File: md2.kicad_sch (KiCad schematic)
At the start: 39 parts, among them IC1 TC74HC4066AP_F_, IC2 TC74HC4066AP_F_, IC3 TC74HC04AP, IC4 TB6643KQ, IC5 TB6643KQ, IC6 TB6643KQ, IC7 TB6643KQ, J1 Conn_01x03_Pin, J10 Conn_01x02_Pin, J11 Conn_01x01_Pin, J2 Conn_01x03_Pin, J3 Conn_01x03_Pin, J4 Conn_01x03_Pin, J5 XT30PW-M, J6 XT30PW-M, J7 XT30PW-M, J8 XT30PW-M, J9 Conn_01x02_Pin, SW1 SW_Push, SW2 SW_Push, SW3 SW_Push, SW4 SW_Push, SW5 SW_Push, SW6 SW_Push, SW7 SW_Push, SW8 SW_Push, SW9 SW_Push, U1 NJM7805FA

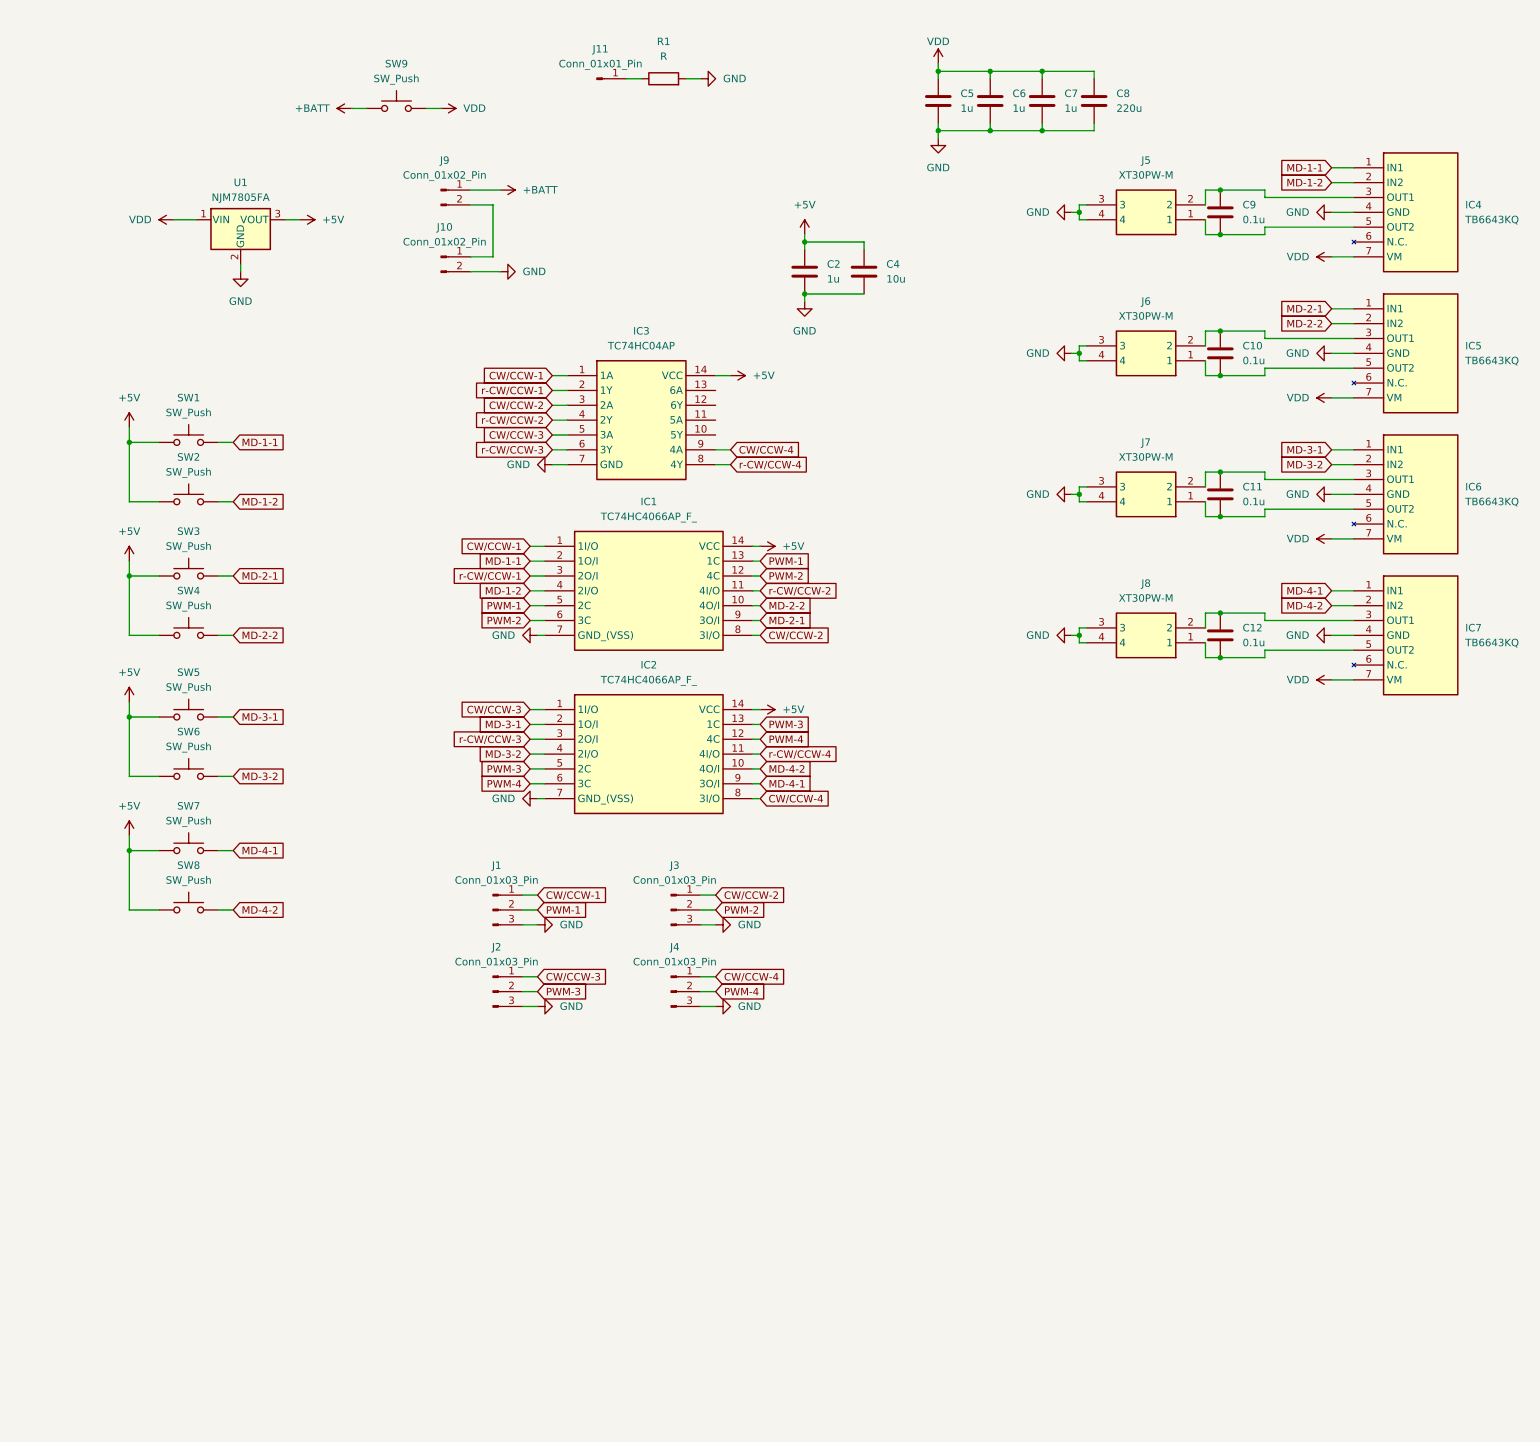
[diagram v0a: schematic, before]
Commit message: Update
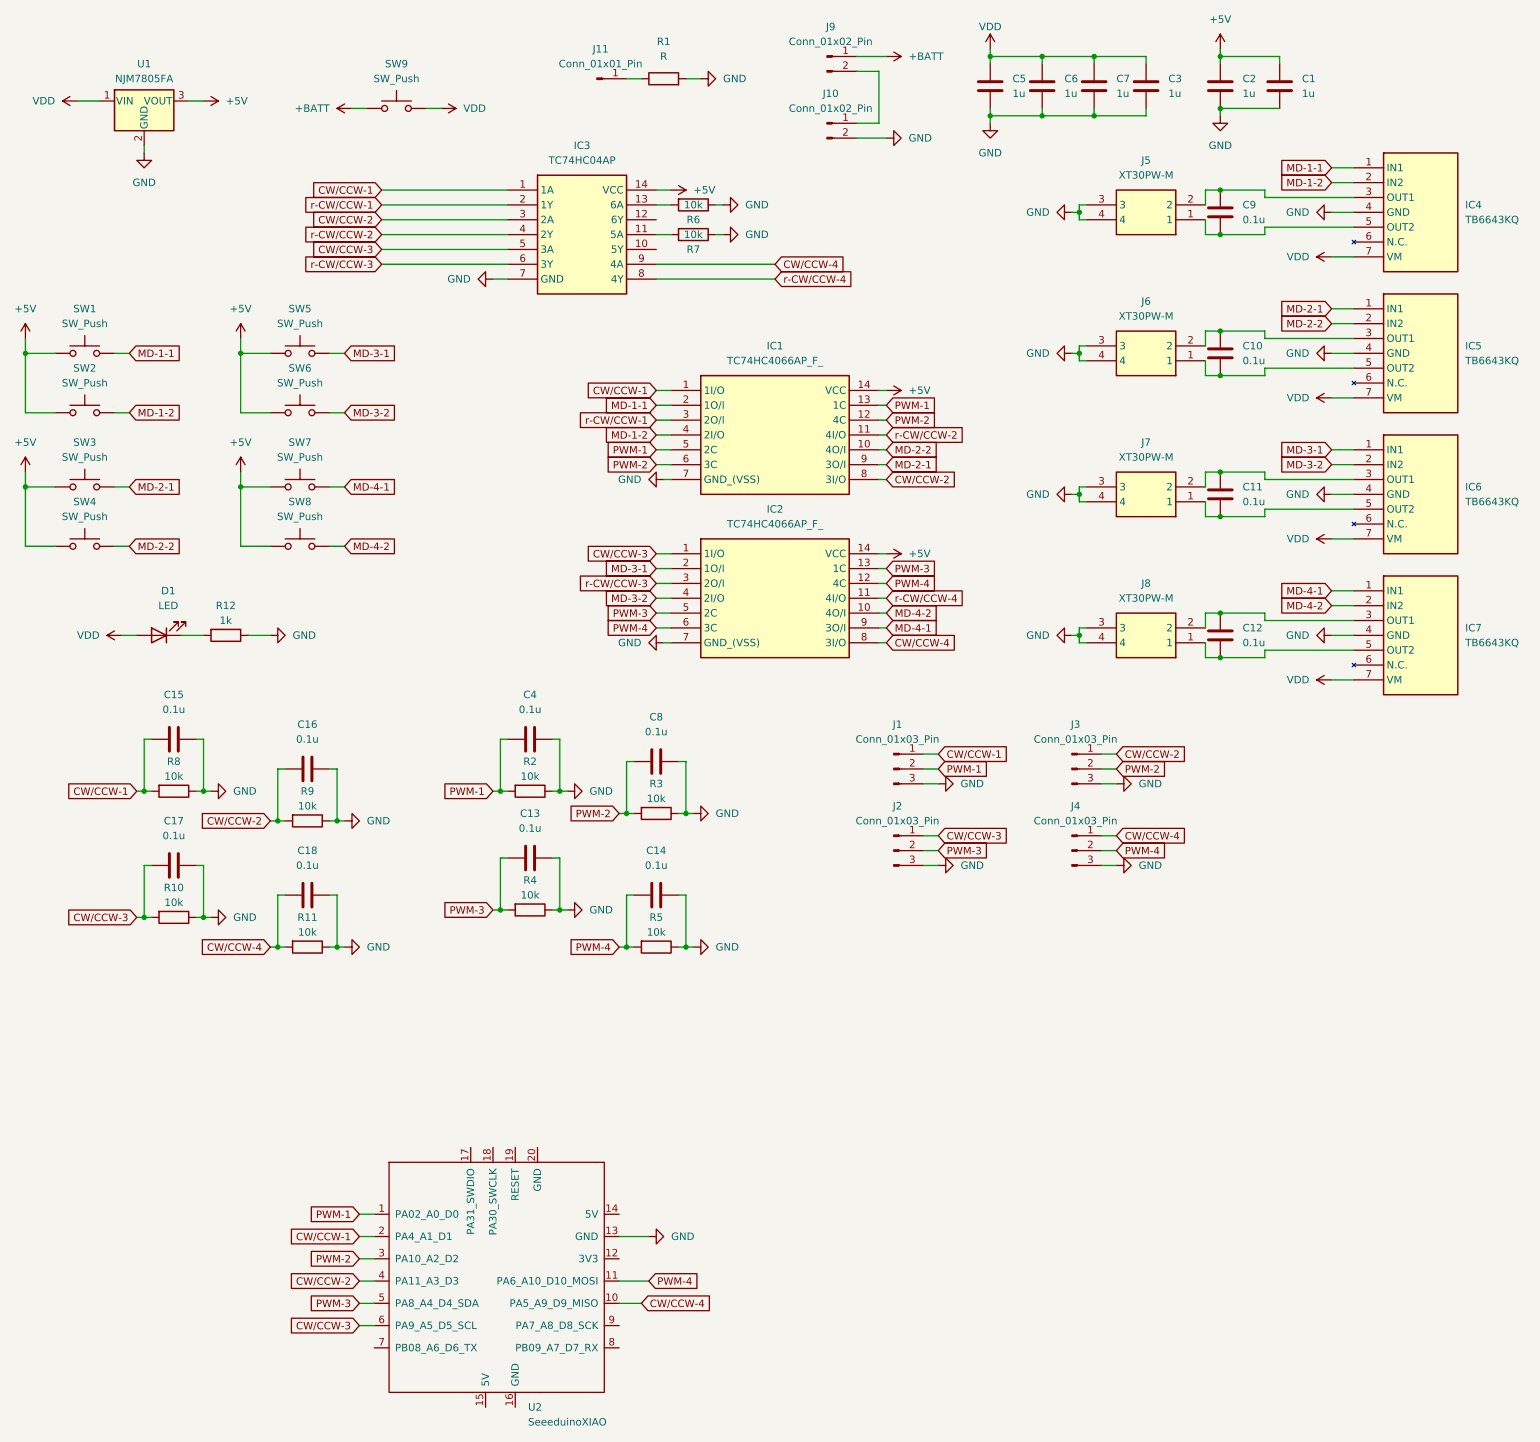
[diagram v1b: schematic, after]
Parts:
- added C1, C3: 1u, Capacitor_THT:C_Disc_D6.0mm_W4.4mm_P5.00mm, symbol Device:C
- added C13, C14, C15, C16, C17, C18: 0.1u, Capacitor_THT:C_Disc_D6.0mm_W4.4mm_P5.00mm, symbol Device:C
- added D1: LED, LED_THT:LED_D3.0mm, symbol Device:LED
- added R10, R11, R2, R3, R4, R5, R6, R7, R8, R9: 10k, Resistor_THT:R_Axial_DIN0207_L6.3mm_D2.5mm_P10.16mm_Horizontal, symbol Device:R
- added R12: 1k, Resistor_THT:R_Axial_DIN0207_L6.3mm_D2.5mm_P10.16mm_Horizontal, symbol Device:R
- added U2: SeeeduinoXIAO, Seeeduino XIAO KICAD:Seeeduino XIAO-MOUDLE14P-2.54-21X17.8MM, symbol Seeeduino XIAO:SeeeduinoXIAO
- C4: value 10u -> 0.1u; footprint Capacitor_THT:CP_Radial_D5.0mm_P2.00mm -> Capacitor_THT:C_Disc_D6.0mm_W4.4mm_P5.00mm
- C8: value 220u -> 0.1u; footprint Capacitor_THT:CP_Radial_D8.0mm_P3.50mm -> Capacitor_THT:C_Disc_D6.0mm_W4.4mm_P5.00mm
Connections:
- net +5V: now also C1.1; no longer C4.1
- net CW/CCW-1: now also C15.1, R8.2, U2.2 (PA4_A1_D1)
- net CW/CCW-2: now also C16.1, R9.2, U2.4 (PA11_A3_D3)
- net CW/CCW-3: now also C17.1, R10.2, U2.6 (PA9_A5_D5_SCL)
- net CW/CCW-4: now also C18.1, R11.2, U2.10 (PA5_A9_D9_MISO)
- net GND: now also C1.2, C13.2, C14.2, C15.2, C16.2, C17.2, C18.2, C3.2, R10.1, R11.1, R12.1, R2.1, R3.1, R4.1, R5.1, R6.1, R7.1, R8.1, R9.1, U2.13 (GND)
- net PWM-1: now also C4.1, R2.2, U2.1 (PA02_A0_D0)
- net PWM-2: now also C8.1, R3.2, U2.3 (PA10_A2_D2)
- net PWM-3: now also C13.1, R4.2, U2.5 (PA8_A4_D4_SDA)
- net PWM-4: now also C14.1, R5.2, U2.11 (PA6_A10_D10_MOSI)
- net VDD: now also C3.1, D1.2 (A); no longer C8.1
- net at IC3.11 (5A): now also R7.2
- net at IC3.13 (6A): now also R6.2
- new net: D1.1 (K), R12.2
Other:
- moved on the sheet: C2, C5, C6, C7, IC1, IC2, IC3, J1, J10, J2, J3, J4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
